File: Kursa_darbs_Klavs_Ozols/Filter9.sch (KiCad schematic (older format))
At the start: 11 parts, among them U10 TL074

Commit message: Shii ir kursa darba 3. iteraacija
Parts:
- C43, C44, C45, C46: footprint (none) -> Capacitors_THT:C_Axial_L5.1mm_D3.1mm_P10.00mm_Horizontal
- R49, R50, R52, R53, R54: footprint (none) -> Resistors_THT:R_Axial_DIN0309_L9.0mm_D3.2mm_P5.08mm_Vertical
- R51: footprint (none) -> Resistors_THT:R_Axial_DIN0414_L11.9mm_D4.5mm_P20.32mm_Horizontal
- U10: footprint (none) -> TL074:DIL14
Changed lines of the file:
@@
 F 0 "U10" H 3950 3500 50  0000 L CNN
 F 1 "TL074" H 3950 3100 50  0000 L CNN
-F 2 "" H 3900 3400 50  0001 C CNN
+F 2 "TL074:DIL14" H 3900 3400 50  0001 C CNN
 F 3 "" H 4000 3500 50  0001 C CNN
 	1    3950 3300
@@
 F 0 "R49" V 2480 3400 50  0000 C CNN
 F 1 "6.8k" V 2400 3400 50  0000 C CNN
-F 2 "" V 2330 3400 50  0001 C CNN
-F 3 "" H 2400 3400 50  0001 C CNN
+F 2 "Resistors_THT:R_Axial_DIN0309_L9.0mm_D3.2mm_P5.08mm_Vertical" V 2330 3400 50  0001 C CNN
+F 3 "https://eu.mouser.com/datasheet/2/219/MOS-16613.pdf" H 2400 3400 50  0001 C CNN
 	1    2400 3400
 	0    1    1    0
@@
 F 0 "R50" V 2730 3200 50  0000 C CNN
 F 1 "5.1k" V 2650 3200 50  0000 C CNN
-F 2 "" V 2580 3200 50  0001 C CNN
-F 3 "" H 2650 3200 50  0001 C CNN
+F 2 "Resistors_THT:R_Axial_DIN0309_L9.0mm_D3.2mm_P5.08mm_Vertical" V 2580 3200 50  0001 C CNN
+F 3 "https://eu.mouser.com/datasheet/2/219/MOS-16613.pdf" H 2650 3200 50  0001 C CNN
 	1    2650 3200
 	1    0    0    -1
@@
 F 0 "C43" H 2975 3500 50  0000 L CNN
 F 1 "470 pF" H 2975 3300 50  0000 L CNN
-F 2 "" H 2988 3250 50  0001 C CNN
-F 3 "" H 2950 3400 50  0001 C CNN
+F 2 "Capacitors_THT:C_Axial_L5.1mm_D3.1mm_P10.00mm_Horizontal" H 2988 3250 50  0001 C CNN
+F 3 "https://eu.mouser.com/datasheet/2/212/KEM_C1046_AXIAL_MOLDED_X7R-1145195.pdf" H 2950 3400 50  0001 C CNN
 	1    2950 3400
 	0    1    1    0
@@
 F 0 "C44" H 2975 3800 50  0000 L CNN
 F 1 "470 pF" H 2975 3600 50  0000 L CNN
-F 2 "" H 2988 3550 50  0001 C CNN
-F 3 "" H 2950 3700 50  0001 C CNN
+F 2 "Capacitors_THT:C_Axial_L5.1mm_D3.1mm_P10.00mm_Horizontal" H 2988 3550 50  0001 C CNN
+F 3 "https://eu.mouser.com/datasheet/2/212/KEM_C1046_AXIAL_MOLDED_X7R-1145195.pdf" H 2950 3700 50  0001 C CNN
 	1    2950 3700
 	0    1    1    0
@@
 F 0 "R51" V 3480 3550 50  0000 C CNN
 F 1 "62k" V 3400 3550 50  0000 C CNN
-F 2 "" V 3330 3550 50  0001 C CNN
-F 3 "" H 3400 3550 50  0001 C CNN
+F 2 "Resistors_THT:R_Axial_DIN0414_L11.9mm_D4.5mm_P20.32mm_Horizontal" V 3330 3550 50  0001 C CNN
+F 3 "https://eu.mouser.com/datasheet/2/219/MOS-16613.pdf" H 3400 3550 50  0001 C CNN
 	1    3400 3550
 	0    1    1    0
@@
 F 0 "R52" V 4980 3300 50  0000 C CNN
 F 1 "6.8k" V 4900 3300 50  0000 C CNN
-F 2 "" V 4830 3300 50  0001 C CNN
-F 3 "" H 4900 3300 50  0001 C CNN
+F 2 "Resistors_THT:R_Axial_DIN0309_L9.0mm_D3.2mm_P5.08mm_Vertical" V 4830 3300 50  0001 C CNN
+F 3 "https://eu.mouser.com/datasheet/2/219/MOS-16613.pdf" H 4900 3300 50  0001 C CNN
 	1    4900 3300
 	0    1    1    0
@@
 F 0 "R53" V 5230 3100 50  0000 C CNN
 F 1 "5.1k" V 5150 3100 50  0000 C CNN
-F 2 "" V 5080 3100 50  0001 C CNN
-F 3 "" H 5150 3100 50  0001 C CNN
+F 2 "Resistors_THT:R_Axial_DIN0309_L9.0mm_D3.2mm_P5.08mm_Vertical" V 5080 3100 50  0001 C CNN
+F 3 "https://eu.mouser.com/datasheet/2/219/MOS-16613.pdf" H 5150 3100 50  0001 C CNN
 	1    5150 3100
 	1    0    0    -1
@@
 F 0 "C45" H 5475 3400 50  0000 L CNN
 F 1 "470 pF" H 5475 3200 50  0000 L CNN
-F 2 "" H 5488 3150 50  0001 C CNN
-F 3 "" H 5450 3300 50  0001 C CNN
+F 2 "Capacitors_THT:C_Axial_L5.1mm_D3.1mm_P10.00mm_Horizontal" H 5488 3150 50  0001 C CNN
+F 3 "https://eu.mouser.com/datasheet/2/212/KEM_C1046_AXIAL_MOLDED_X7R-1145195.pdf" H 5450 3300 50  0001 C CNN
 	1    5450 3300
 	0    1    1    0
@@
 F 0 "C46" H 5475 3700 50  0000 L CNN
 F 1 "470 pF" H 5475 3500 50  0000 L CNN
-F 2 "" H 5488 3450 50  0001 C CNN
-F 3 "" H 5450 3600 50  0001 C CNN
+F 2 "Capacitors_THT:C_Axial_L5.1mm_D3.1mm_P10.00mm_Horizontal" H 5488 3450 50  0001 C CNN
+F 3 "https://eu.mouser.com/datasheet/2/212/KEM_C1046_AXIAL_MOLDED_X7R-1145195.pdf" H 5450 3600 50  0001 C CNN
 	1    5450 3600
 	0    1    1    0
@@
 F 0 "R54" V 5980 3450 50  0000 C CNN
 F 1 "62k" V 5900 3450 50  0000 C CNN
-F 2 "" V 5830 3450 50  0001 C CNN
-F 3 "" H 5900 3450 50  0001 C CNN
+F 2 "Resistors_THT:R_Axial_DIN0309_L9.0mm_D3.2mm_P5.08mm_Vertical" V 5830 3450 50  0001 C CNN
+F 3 "https://eu.mouser.com/datasheet/2/219/MOS-16613.pdf" H 5900 3450 50  0001 C CNN
 	1    5900 3450
 	0    1    1    0
@@
 F 0 "U10" H 6450 3400 50  0000 L CNN
 F 1 "TL074" H 6450 3000 50  0000 L CNN
-F 2 "" H 6400 3300 50  0001 C CNN
+F 2 "TL074:DIL14" H 6400 3300 50  0001 C CNN
 F 3 "" H 6500 3400 50  0001 C CNN
 	2    6450 3200

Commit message: Kursa darba plates 4. iteraacija
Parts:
- R51: footprint Resistors_THT:R_Axial_DIN0414_L11.9mm_D4.5mm_P20.32mm_Horizontal -> Resistors_THT:R_Axial_DIN0309_L9.0mm_D3.2mm_P5.08mm_Vertical
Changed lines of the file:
@@
 F 0 "R51" V 3480 3550 50  0000 C CNN
 F 1 "62k" V 3400 3550 50  0000 C CNN
-F 2 "Resistors_THT:R_Axial_DIN0414_L11.9mm_D4.5mm_P20.32mm_Horizontal" V 3330 3550 50  0001 C CNN
+F 2 "Resistors_THT:R_Axial_DIN0309_L9.0mm_D3.2mm_P5.08mm_Vertical" V 3330 3550 50  0001 C CNN
 F 3 "https://eu.mouser.com/datasheet/2/219/MOS-16613.pdf" H 3400 3550 50  0001 C CNN
 	1    3400 3550

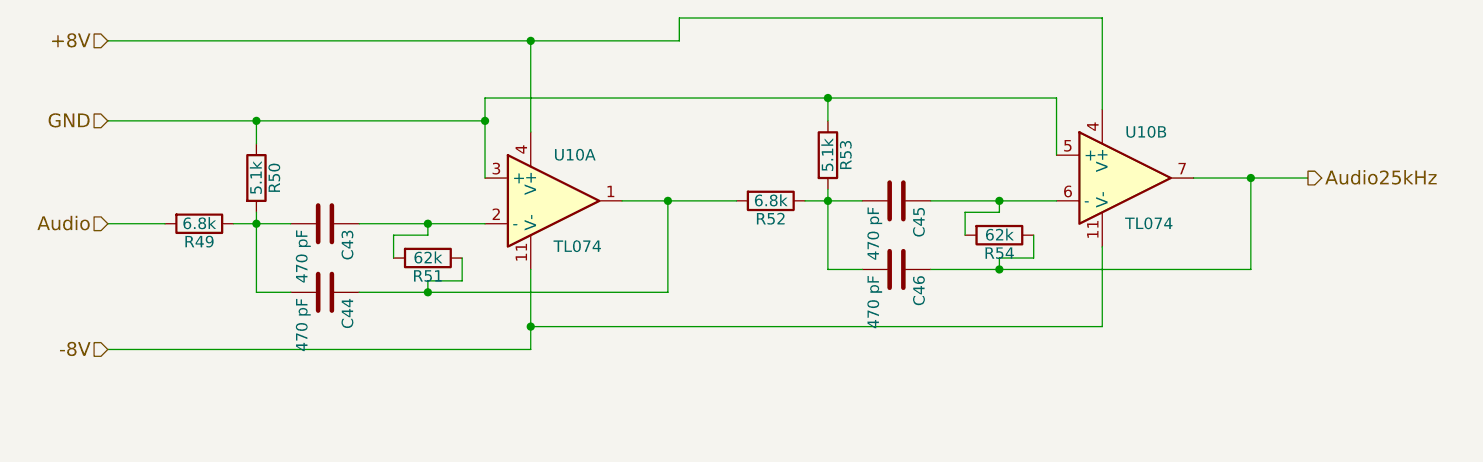
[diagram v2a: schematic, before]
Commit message: Shiii ir 5. iteraacija manai platei - layouts
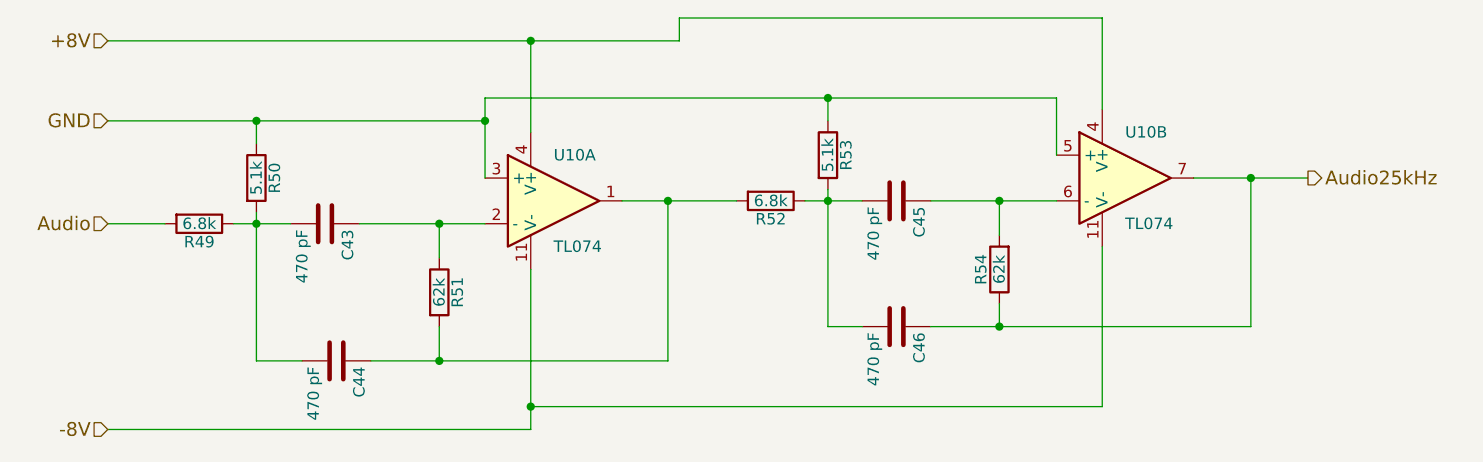
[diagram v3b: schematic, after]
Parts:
- C43, C44, C45, C46: footprint Capacitors_THT:C_Axial_L5.1mm_D3.1mm_P10.00mm_Horizontal -> Capacitors_SMD:C_0805_HandSoldering
- R49, R50, R51, R52, R53, R54: footprint Resistors_THT:R_Axial_DIN0309_L9.0mm_D3.2mm_P5.08mm_Vertical -> Resistors_SMD:R_0805_HandSoldering
- U10: footprint TL074:DIL14 -> TL074:SO14
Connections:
- net at C44.1, R52.2, U10.1: now also R51.2; no longer R51.1
- net at C43.1, U10.2 (-): now also R51.1; no longer R51.2
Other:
- moved on the sheet: C44, C46, R51, R54
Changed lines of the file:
@@
 EESchema Schematic File Version 2
+LIBS:Kursa_darbs_Klavs_Ozols-rescue
 LIBS:power
 LIBS:device
@@
 F 0 "U10" H 3950 3500 50  0000 L CNN
 F 1 "TL074" H 3950 3100 50  0000 L CNN
-F 2 "TL074:DIL14" H 3900 3400 50  0001 C CNN
+F 2 "TL074:SO14" H 3900 3400 50  0001 C CNN
 F 3 "" H 4000 3500 50  0001 C CNN
 	1    3950 3300
@@
 F 0 "R49" V 2480 3400 50  0000 C CNN
 F 1 "6.8k" V 2400 3400 50  0000 C CNN
-F 2 "Resistors_THT:R_Axial_DIN0309_L9.0mm_D3.2mm_P5.08mm_Vertical" V 2330 3400 50  0001 C CNN
-F 3 "https://eu.mouser.com/datasheet/2/219/MOS-16613.pdf" H 2400 3400 50  0001 C CNN
+F 2 "Resistors_SMD:R_0805_HandSoldering" V 2330 3400 50  0001 C CNN
+F 3 "https://eu.mouser.com/datasheet/2/219/RN73-11994.pdf" H 2400 3400 50  0001 C CNN
 	1    2400 3400
 	0    1    1    0
@@
 F 0 "R50" V 2730 3200 50  0000 C CNN
 F 1 "5.1k" V 2650 3200 50  0000 C CNN
-F 2 "Resistors_THT:R_Axial_DIN0309_L9.0mm_D3.2mm_P5.08mm_Vertical" V 2580 3200 50  0001 C CNN
-F 3 "https://eu.mouser.com/datasheet/2/219/MOS-16613.pdf" H 2650 3200 50  0001 C CNN
+F 2 "Resistors_SMD:R_0805_HandSoldering" V 2580 3200 50  0001 C CNN
+F 3 "https://eu.mouser.com/datasheet/2/219/RN73-11994.pdf" H 2650 3200 50  0001 C CNN
 	1    2650 3200
 	1    0    0    -1
@@
 F 0 "C43" H 2975 3500 50  0000 L CNN
 F 1 "470 pF" H 2975 3300 50  0000 L CNN
-F 2 "Capacitors_THT:C_Axial_L5.1mm_D3.1mm_P10.00mm_Horizontal" H 2988 3250 50  0001 C CNN
+F 2 "Capacitors_SMD:C_0805_HandSoldering" H 2988 3250 50  0001 C CNN
 F 3 "https://eu.mouser.com/datasheet/2/212/KEM_C1046_AXIAL_MOLDED_X7R-1145195.pdf" H 2950 3400 50  0001 C CNN
 	1    2950 3400
@@
 L C C44
 U 1 1 5B022A39
-P 2950 3700
-F 0 "C44" H 2975 3800 50  0000 L CNN
-F 1 "470 pF" H 2975 3600 50  0000 L CNN
-F 2 "Capacitors_THT:C_Axial_L5.1mm_D3.1mm_P10.00mm_Horizontal" H 2988 3550 50  0001 C CNN
-F 3 "https://eu.mouser.com/datasheet/2/212/KEM_C1046_AXIAL_MOLDED_X7R-1145195.pdf" H 2950 3700 50  0001 C CNN
-	1    2950 3700
+P 3000 4000
+F 0 "C44" H 3025 4100 50  0000 L CNN
+F 1 "470 pF" H 3025 3900 50  0000 L CNN
+F 2 "Capacitors_SMD:C_0805_HandSoldering" H 3038 3850 50  0001 C CNN
+F 3 "https://eu.mouser.com/datasheet/2/212/KEM_C1046_AXIAL_MOLDED_X7R-1145195.pdf" H 3000 4000 50  0001 C CNN
+	1    3000 4000
 	0    1    1    0
 $EndComp
@@
 L R R51
 U 1 1 5B022AB9
-P 3400 3550
-F 0 "R51" V 3480 3550 50  0000 C CNN
-F 1 "62k" V 3400 3550 50  0000 C CNN
-F 2 "Resistors_THT:R_Axial_DIN0309_L9.0mm_D3.2mm_P5.08mm_Vertical" V 3330 3550 50  0001 C CNN
-F 3 "https://eu.mouser.com/datasheet/2/219/MOS-16613.pdf" H 3400 3550 50  0001 C CNN
-	1    3400 3550
-	0    1    1    0
+P 3450 3700
+F 0 "R51" V 3530 3700 50  0000 C CNN
+F 1 "62k" V 3450 3700 50  0000 C CNN
+F 2 "Resistors_SMD:R_0805_HandSoldering" V 3380 3700 50  0001 C CNN
+F 3 "https://eu.mouser.com/datasheet/2/219/RN73-11994.pdf" H 3450 3700 50  0001 C CNN
+	1    3450 3700
+	1    0    0    -1
 $EndComp
 Text HLabel 2000 2950 0    60   Input ~ 0
@@
 Text HLabel 2000 2600 0    60   Input ~ 0
 +8V
-Text HLabel 2000 3950 0    60   Input ~ 0
+Text HLabel 2000 4300 0    60   Input ~ 0
 -8V
 $Comp
@@
 F 0 "R52" V 4980 3300 50  0000 C CNN
 F 1 "6.8k" V 4900 3300 50  0000 C CNN
-F 2 "Resistors_THT:R_Axial_DIN0309_L9.0mm_D3.2mm_P5.08mm_Vertical" V 4830 3300 50  0001 C CNN
-F 3 "https://eu.mouser.com/datasheet/2/219/MOS-16613.pdf" H 4900 3300 50  0001 C CNN
+F 2 "Resistors_SMD:R_0805_HandSoldering" V 4830 3300 50  0001 C CNN
+F 3 "https://eu.mouser.com/datasheet/2/219/RN73-11994.pdf" H 4900 3300 50  0001 C CNN
 	1    4900 3300
 	0    1    1    0
@@
 F 0 "R53" V 5230 3100 50  0000 C CNN
 F 1 "5.1k" V 5150 3100 50  0000 C CNN
-F 2 "Resistors_THT:R_Axial_DIN0309_L9.0mm_D3.2mm_P5.08mm_Vertical" V 5080 3100 50  0001 C CNN
-F 3 "https://eu.mouser.com/datasheet/2/219/MOS-16613.pdf" H 5150 3100 50  0001 C CNN
+F 2 "Resistors_SMD:R_0805_HandSoldering" V 5080 3100 50  0001 C CNN
+F 3 "https://eu.mouser.com/datasheet/2/219/RN73-11994.pdf" H 5150 3100 50  0001 C CNN
 	1    5150 3100
 	1    0    0    -1
@@
 F 0 "C45" H 5475 3400 50  0000 L CNN
 F 1 "470 pF" H 5475 3200 50  0000 L CNN
-F 2 "Capacitors_THT:C_Axial_L5.1mm_D3.1mm_P10.00mm_Horizontal" H 5488 3150 50  0001 C CNN
+F 2 "Capacitors_SMD:C_0805_HandSoldering" H 5488 3150 50  0001 C CNN
 F 3 "https://eu.mouser.com/datasheet/2/212/KEM_C1046_AXIAL_MOLDED_X7R-1145195.pdf" H 5450 3300 50  0001 C CNN
 	1    5450 3300
@@
 L C C46
 U 1 1 5B022D5C
-P 5450 3600
-F 0 "C46" H 5475 3700 50  0000 L CNN
-F 1 "470 pF" H 5475 3500 50  0000 L CNN
-F 2 "Capacitors_THT:C_Axial_L5.1mm_D3.1mm_P10.00mm_Horizontal" H 5488 3450 50  0001 C CNN
-F 3 "https://eu.mouser.com/datasheet/2/212/KEM_C1046_AXIAL_MOLDED_X7R-1145195.pdf" H 5450 3600 50  0001 C CNN
-	1    5450 3600
+P 5450 3850
+F 0 "C46" H 5475 3950 50  0000 L CNN
+F 1 "470 pF" H 5475 3750 50  0000 L CNN
+F 2 "Capacitors_SMD:C_0805_HandSoldering" H 5488 3700 50  0001 C CNN
+F 3 "https://eu.mouser.com/datasheet/2/212/KEM_C1046_AXIAL_MOLDED_X7R-1145195.pdf" H 5450 3850 50  0001 C CNN
+	1    5450 3850
 	0    1    1    0
 $EndComp
@@
 L R R54
 U 1 1 5B022D62
-P 5900 3450
-F 0 "R54" V 5980 3450 50  0000 C CNN
-F 1 "62k" V 5900 3450 50  0000 C CNN
-F 2 "Resistors_THT:R_Axial_DIN0309_L9.0mm_D3.2mm_P5.08mm_Vertical" V 5830 3450 50  0001 C CNN
-F 3 "https://eu.mouser.com/datasheet/2/219/MOS-16613.pdf" H 5900 3450 50  0001 C CNN
-	1    5900 3450
-	0    1    1    0
+P 5900 3600
+F 0 "R54" V 5980 3600 50  0000 C CNN
+F 1 "62k" V 5900 3600 50  0000 C CNN
+F 2 "Resistors_SMD:R_0805_HandSoldering" V 5830 3600 50  0001 C CNN
+F 3 "https://eu.mouser.com/datasheet/2/219/RN73-11994.pdf" H 5900 3600 50  0001 C CNN
+	1    5900 3600
+	-1   0    0    1
 $EndComp
 Text HLabel 7250 3200 2    60   Output ~ 0
@@
 F 0 "U10" H 6450 3400 50  0000 L CNN
 F 1 "TL074" H 6450 3000 50  0000 L CNN
-F 2 "TL074:DIL14" H 6400 3300 50  0001 C CNN
+F 2 "TL074:SO14" H 6400 3300 50  0001 C CNN
 F 3 "" H 6500 3400 50  0001 C CNN
 	2    6450 3200
@@
 Wire Wire Line
 	3100 3400 3650 3400
-Connection ~ 3400 3400
-Wire Wire Line
-	3100 3700 4450 3700
 Wire Wire Line
 	2550 3400 2800 3400
 Wire Wire Line
-	2650 3350 2650 3700
+	2650 3350 2650 4000
 Connection ~ 2650 3400
-Wire Wire Line
-	2650 3700 2800 3700
 Wire Wire Line
 	2000 2950 3650 2950
@@
 	2000 2600 4500 2600
 Wire Wire Line
-	3850 3600 3850 3950
-Wire Wire Line
-	3850 3950 2000 3950
+	3850 3600 3850 4300
+Wire Wire Line
+	3850 4300 2000 4300
 Wire Wire Line
 	2250 3400 2000 3400
@@
 Connection ~ 5900 3300
 Wire Wire Line
-	5600 3600 7000 3600
-Wire Wire Line
 	5050 3300 5300 3300
 Wire Wire Line
-	5150 3250 5150 3600
+	5150 3250 5150 3850
 Connection ~ 5150 3300
-Wire Wire Line
-	5150 3600 5300 3600
 Wire Wire Line
 	3650 2850 6150 2850
@@
 	6350 2500 4500 2500
 Wire Wire Line
-	6350 3850 6350 3500
-Wire Wire Line
-	3850 3850 6350 3850
+	6350 3500 6350 4200
+Wire Wire Line
+	6350 4200 3850 4200
 Wire Wire Line
 	4250 3300 4750 3300
-Connection ~ 3850 3850
-Wire Wire Line
-	4450 3700 4450 3300
+Connection ~ 3850 4200
+Wire Wire Line
+	4450 3300 4450 4000
 Connection ~ 4450 3300
-Connection ~ 3400 3700
 Connection ~ 3650 2950
 Wire Wire Line
@@
 	7250 3200 6750 3200
 Wire Wire Line
-	7000 3600 7000 3200
+	7000 3850 7000 3200
 Connection ~ 7000 3200
-Connection ~ 5900 3600
-Wire Wire Line
-	3400 3400 3400 3450
-Wire Wire Line
-	3400 3450 3250 3450
-Wire Wire Line
-	3250 3450 3250 3550
-Wire Wire Line
-	3550 3550 3550 3650
-Wire Wire Line
-	3550 3650 3400 3650
-Wire Wire Line
-	3400 3650 3400 3700
-Wire Wire Line
-	5750 3450 5750 3350
-Wire Wire Line
-	5750 3350 5900 3350
-Wire Wire Line
-	5900 3350 5900 3300
-Wire Wire Line
-	6050 3450 6050 3550
-Wire Wire Line
-	6050 3550 5900 3550
-Wire Wire Line
-	5900 3550 5900 3600
+Wire Wire Line
+	5150 3850 5300 3850
+Wire Wire Line
+	5900 3300 5900 3450
+Wire Wire Line
+	5900 3750 5900 3850
+Wire Wire Line
+	5600 3850 7000 3850
+Connection ~ 5900 3850
+Wire Wire Line
+	2650 4000 2850 4000
+Wire Wire Line
+	4450 4000 3150 4000
+Wire Wire Line
+	3450 3850 3450 4000
+Connection ~ 3450 4000
+Wire Wire Line
+	3450 3550 3450 3400
+Connection ~ 3450 3400
 $EndSCHEMATC
